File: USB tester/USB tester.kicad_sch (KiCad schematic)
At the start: 9 parts, among them J3 USB_A

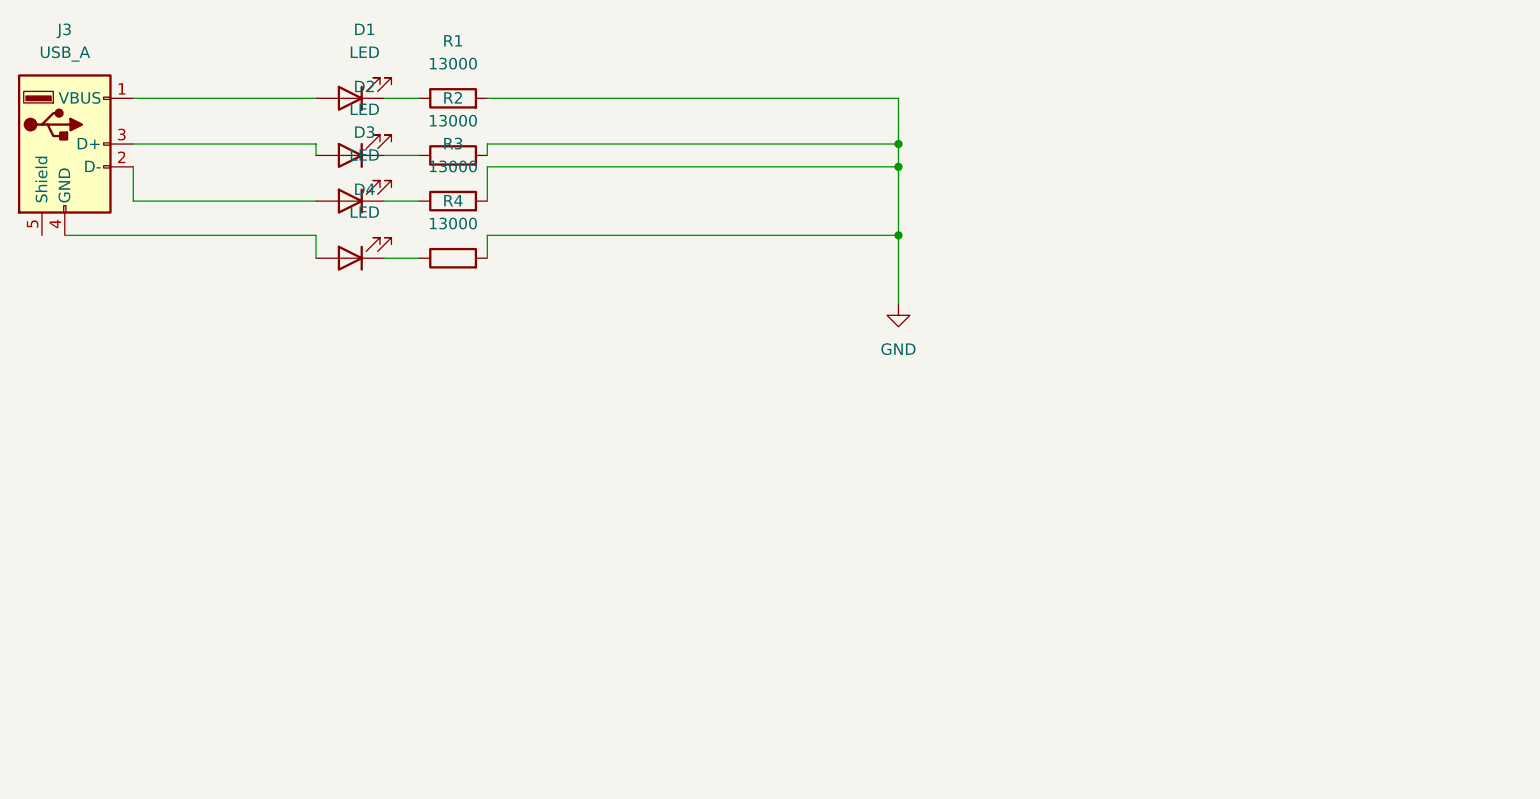
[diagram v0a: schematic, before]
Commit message: update
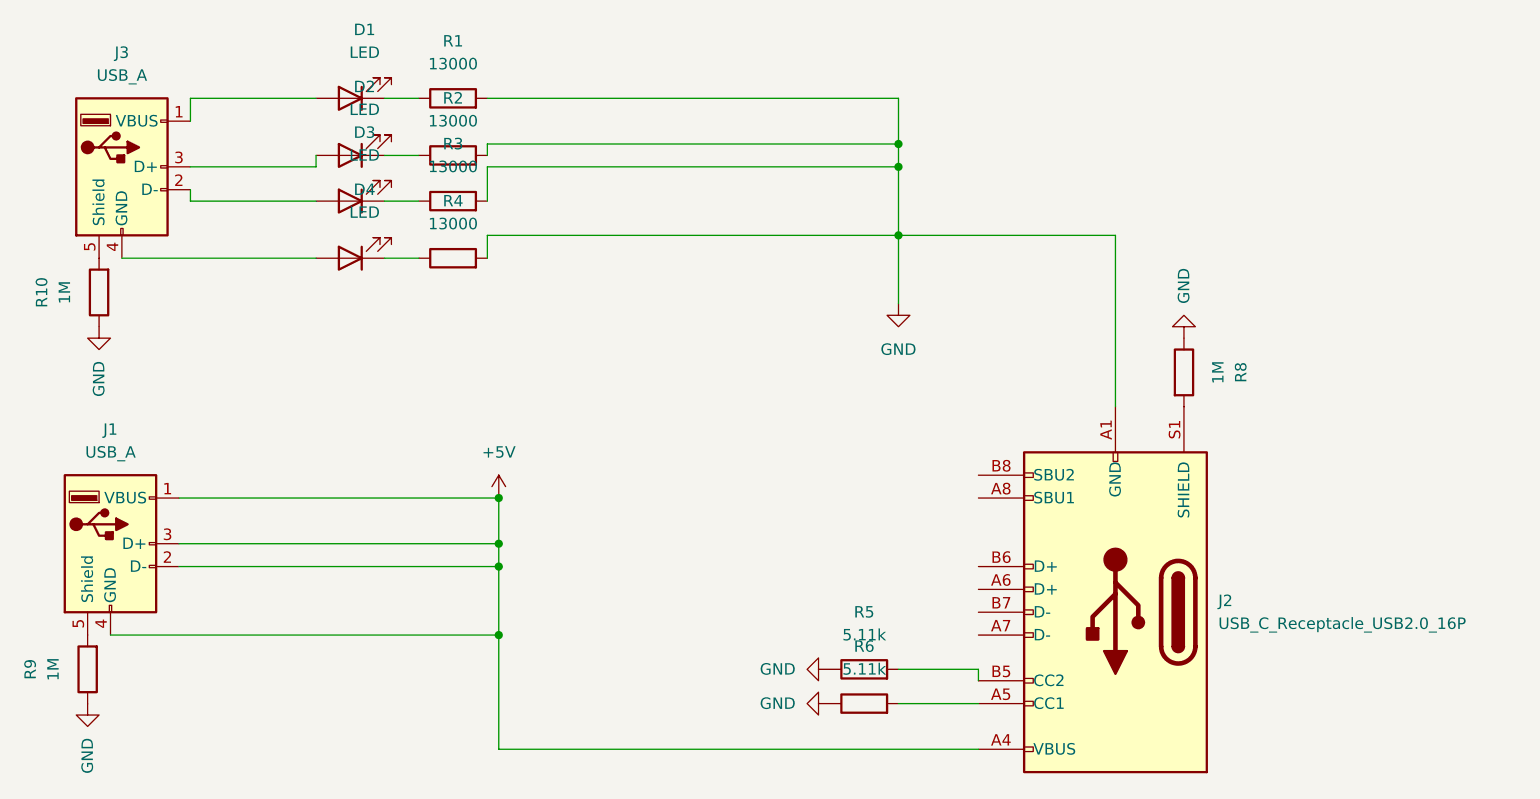
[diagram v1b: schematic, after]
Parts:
- added J1: USB_A, Connector_USB:USB_A_Receptacle_GCT_USB1046, symbol Connector:USB_A
- added J2: USB_C_Receptacle_USB2.0_16P, Connector_USB:USB_C_Receptacle_G-Switch_GT-USB-7010ASV, symbol Connector:USB_C_Receptacle_USB2.0_16P
- added R10, R8, R9: 1M, Resistor_SMD:R_0805_2012Metric, symbol Device:R
- added R5, R6: 5.11k, Resistor_SMD:R_0805_2012Metric, symbol Device:R
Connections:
- net GND: now also J2.A1 (GND), J2.A12 (GND), J2.B1 (GND), J2.B12 (GND), R10.1, R5.1, R6.1, R8.1, R9.1
- net at J3.5 (Shield): now also R10.2
- new net: J2.A5 (CC1), R6.2
- new net: J2.B5 (CC2), R5.2
- new net: J2.S1 (SHIELD), R8.2
- new net: J1.5 (Shield), R9.2
- new net +5V: J1.1 (VBUS), J1.2 (D-), J1.3 (D+), J1.4 (GND), J2.A4 (VBUS), J2.A9 (VBUS), J2.B4 (VBUS), J2.B9 (VBUS)
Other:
- moved on the sheet: J3
